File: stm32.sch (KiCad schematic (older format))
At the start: 39 parts, among them J2 MINI-USB-5P-3400020P1, J3 Conn_02x05_Odd_Even, U1 STM32F767VITx, U30 LM2937, X1 8MHz, X2 32.768K

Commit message: fix usb
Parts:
- removed J2: MINI-USB-5P-3400020P1, Connector_USB:USB_Micro-B_Molex-105133-0031, symbol BOSCH_154_PIN:MINI-USB-5P-3400020P1
- removed R102: 10K, Resistor_SMD:R_0805_2012Metric_Pad1.15x1.40mm_HandSolder, symbol ME7_Universal-rescue:R-adc_amp_dividor-cache-ME7_Universal-rescue
- removed R103: 680, Resistor_SMD:R_0805_2012Metric_Pad1.15x1.40mm_HandSolder, symbol ME7_Universal-rescue:R-adc_amp_dividor-cache-ME7_Universal-rescue
- added J2: USB_B_Micro, symbol Connector:USB_B_Micro
- added R102: 10k, symbol Device:R
- added R103: 680, symbol Device:R
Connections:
- wire segments 74 -> 75
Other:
- moved on the sheet: C75, D17, R100
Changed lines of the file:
@@
-$EndComp
-$Comp
-L BOSCH_154_PIN:MINI-USB-5P-3400020P1 J2
-U 1 1 52D197D7
-P 11600 4250
-F 0 "J2" H 11325 4600 60  0000 C CNN
-F 1 "MINI-USB-5P-3400020P1" H 11600 4700 60  0001 C CNN
-F 2 "Connector_USB:USB_Micro-B_Molex-105133-0031" V 430 1700 60  0001 C CNN
-F 3 "" H 11600 4250 60  0001 C CNN
-F 4 "stm32f407_board" H 11950 1275 60  0001 C CNN "PageName"
-F 5 "MOUSER" H -6050 -2300 50  0001 C CNN "VEND"
-F 6 "MOLEX" H -6050 -2300 50  0001 C CNN "Manufacturer"
-F 7 "105133-0031" H -6050 -2300 50  0001 C CNN "Part #"
-F 8 "538-105133-0031" H -6050 -2300 50  0001 C CNN "VEND#"
-	1    11600 4250
-	1    0    0    -1
 $EndComp
 $Comp
 L power:GND #PWR0141
 U 1 1 5CE96D9C
-P 12100 4600
-F 0 "#PWR0141" H 12100 4600 30  0001 C CNN
-F 1 "GND" H 12100 4530 30  0001 C CNN
-F 2 "" H 12100 4600 60  0000 C CNN
-F 3 "" H 12100 4600 60  0000 C CNN
-	1    12100 4600
+P 11500 4750
+F 0 "#PWR0141" H 11500 4750 30  0001 C CNN
+F 1 "GND" H 11500 4680 30  0001 C CNN
+F 2 "" H 11500 4750 60  0000 C CNN
+F 3 "" H 11500 4750 60  0000 C CNN
+	1    11500 4750
 	1    0    0    -1
 $EndComp
@@
 L power:GND #PWR0144
 U 1 1 5C5BFED2
-P 12950 5000
-F 0 "#PWR0144" H 12950 5000 30  0001 C CNN
-F 1 "GND" H 12950 4930 30  0001 C CNN
-F 2 "" H 12950 5000 60  0001 C CNN
-F 3 "" H 12950 5000 60  0001 C CNN
-	1    12950 5000
-	1    0    0    -1
-$EndComp
-Text Notes 12800 5800 0    60   ~ 12
+P 12950 5050
+F 0 "#PWR0144" H 12950 5050 30  0001 C CNN
+F 1 "GND" H 12950 4980 30  0001 C CNN
+F 2 "" H 12950 5050 60  0001 C CNN
+F 3 "" H 12950 5050 60  0001 C CNN
+	1    12950 5050
+	1    0    0    -1
+$EndComp
+Text Notes 11750 6650 0    60   ~ 12
 SWD
 Text Label 12100 6300 0    60   ~ 12
@@
 Text Notes 12450 5250 0    60   ~ 12
 diodes schottky 20V 1A SD0805S020S1R0
-Text Label 13450 4300 0    60   ~ 12
+Text Label 13450 4400 0    60   ~ 12
 PA10
-Text Label 14250 4000 0    60   ~ 12
+Text Label 14150 4000 0    60   ~ 12
 PA9
 Text HLabel 6600 2000 2    60   Input ~ 12
@@
 Text HLabel 14150 3400 0    60   Input ~ 12
 5V
-Text HLabel 12200 4400 2    60   Input ~ 12
+Text HLabel 11500 4650 2    60   Input ~ 12
 GND
-Text Label 11800 4500 0    60   ~ 12
+Text Label 11400 4700 2    60   ~ 12
 shield
 Wire Wire Line
@@
 Wire Wire Line
 	12300 3800 12400 3800
-$Comp
-L ME7_Universal-rescue:R-adc_amp_dividor-cache-ME7_Universal-rescue R?
-U 1 1 5C7B03F9
-P 15800 3400
-AR Path="/5C7B03F9" Ref="R?"  Part="1"
-AR Path="/5D0250FB/5C7B03F9" Ref="R103"  Part="1"
-F 0 "R103" V 15700 3400 40  0000 C CNN
-F 1 "680" V 15800 3400 40  0000 C CNN
-F 2 "Resistor_SMD:R_0805_2012Metric_Pad1.15x1.40mm_HandSolder" V 15730 3400 30  0001 C CNN
-F 3 "" H 15800 3400 30  0000 C CNN
-	1    15800 3400
-	0    1    1    0
-$EndComp
 Wire Wire Line
 	14900 3400 15200 3400
@@
 L Power_Protection:ESDA6V1BC6 D17
 U 1 1 5C850928
-P 12950 4700
-F 0 "D17" H 13280 4746 50  0000 L CNN
-F 1 "ESDA6V1BC6" H 13280 4655 50  0000 L CNN
-F 2 "Package_TO_SOT_SMD:SOT-23-6" H 12950 4350 50  0001 C CNN
-F 3 "http://www.st.com/content/ccc/resource/technical/document/datasheet/21/07/21/e3/a8/df/42/a2/CD00001906.pdf/files/CD00001906.pdf/jcr:content/translations/en.CD00001906.pdf" V 12950 4700 50  0001 C CNN
-	1    12950 4700
-	1    0    0    -1
-$EndComp
-Text Label 13450 4100 0    60   ~ 12
+P 12950 4750
+F 0 "D17" H 13280 4796 50  0000 L CNN
+F 1 "ESDA6V1BC6" H 13280 4705 50  0000 L CNN
+F 2 "Package_TO_SOT_SMD:SOT-23-6" H 12950 4400 50  0001 C CNN
+F 3 "http://www.st.com/content/ccc/resource/technical/document/datasheet/21/07/21/e3/a8/df/42/a2/CD00001906.pdf/files/CD00001906.pdf/jcr:content/translations/en.CD00001906.pdf" V 12950 4750 50  0001 C CNN
+	1    12950 4750
+	1    0    0    -1
+$EndComp
+Text Label 13450 4300 0    60   ~ 12
 PA11
 Text Label 13450 4200 0    60   ~ 12
@@
 	11800 4200 13050 4200
 Wire Wire Line
-	11800 4100 12850 4100
-Wire Wire Line
-	11800 4300 13150 4300
-Wire Wire Line
 	11875 4000 12750 4000
-Wire Wire Line
-	12750 4400 12750 4000
 Connection ~ 12750 4000
-Wire Wire Line
-	12850 4400 12850 4100
-Connection ~ 12850 4100
-Wire Wire Line
-	12850 4100 13450 4100
-Wire Wire Line
-	13050 4400 13050 4200
 Connection ~ 13050 4200
 Wire Wire Line
 	13050 4200 13450 4200
-Wire Wire Line
-	13150 4400 13150 4300
-Connection ~ 13150 4300
-Wire Wire Line
-	13150 4300 13450 4300
-$Comp
-L ME7_Universal-rescue:R-adc_amp_dividor-cache-ME7_Universal-rescue R?
-U 1 1 5C920125
-P 14000 4000
-AR Path="/5C920125" Ref="R?"  Part="1"
-AR Path="/5D0250FB/5C920125" Ref="R102"  Part="1"
-F 0 "R102" V 13900 4000 40  0000 C CNN
-F 1 "10K" V 14000 4000 40  0000 C CNN
-F 2 "Resistor_SMD:R_0805_2012Metric_Pad1.15x1.40mm_HandSolder" V 13930 4000 30  0001 C CNN
-F 3 "" H 14000 4000 30  0000 C CNN
-	1    14000 4000
-	0    1    1    0
-$EndComp
-Text Label 12150 4100 0    60   ~ 0
+Text Label 12150 4300 0    60   ~ 0
 D-
 Text Label 12150 4200 0    60   ~ 0
@@
 Wire Wire Line
 	13150 4000 13750 4000
-Wire Wire Line
-	11800 4400 12100 4400
-Wire Wire Line
-	12100 4400 12100 4600
-Connection ~ 12100 4400
-Wire Wire Line
-	12100 4400 12200 4400
 Wire Wire Line
 	14300 3400 14150 3400
@@
 $EndComp
 Wire Wire Line
-	11600 4650 11800 4650
-Wire Wire Line
-	11800 4500 11800 4650
-Wire Wire Line
-	11800 4650 11800 4750
-Connection ~ 11800 4650
+	11200 4750 11400 4750
+Wire Wire Line
+	11400 4600 11400 4750
+Wire Wire Line
+	11400 4750 11400 4850
+Connection ~ 11400 4750
 $Comp
 L power:GND #PWR0138
 U 1 1 5C5BFED7
-P 11600 4950
-F 0 "#PWR0138" H 11600 4950 30  0001 C CNN
-F 1 "GND" H 11600 4880 30  0001 C CNN
-F 2 "" H 11600 4950 60  0001 C CNN
-F 3 "" H 11600 4950 60  0001 C CNN
-	1    11600 4950
+P 11200 5050
+F 0 "#PWR0138" H 11200 5050 30  0001 C CNN
+F 1 "GND" H 11200 4980 30  0001 C CNN
+F 2 "" H 11200 5050 60  0001 C CNN
+F 3 "" H 11200 5050 60  0001 C CNN
+	1    11200 5050
 	1    0    0    -1
 $EndComp
@@
 L Device:R R100
 U 1 1 5D0251FB
-P 11600 4800
-F 0 "R100" V 11680 4800 50  0000 C CNN
-F 1 "100k" V 11600 4800 50  0000 C CNN
-F 2 "Resistor_SMD:R_0805_2012Metric_Pad1.15x1.40mm_HandSolder" H 11600 4800 60  0001 C CNN
-F 3 "" H 11600 4800 60  0001 C CNN
-F 4 "stm32f407_board" H 11950 1175 60  0001 C CNN "PageName"
-F 5 "MOUSER" H -6050 -2300 50  0001 C CNN "VEND"
-	1    11600 4800
+P 11200 4900
+F 0 "R100" V 11280 4900 50  0000 C CNN
+F 1 "100k" V 11200 4900 50  0000 C CNN
+F 2 "Resistor_SMD:R_0805_2012Metric_Pad1.15x1.40mm_HandSolder" H 11200 4900 60  0001 C CNN
+F 3 "" H 11200 4900 60  0001 C CNN
+F 4 "stm32f407_board" H 11550 1275 60  0001 C CNN "PageName"
+F 5 "MOUSER" H -6450 -2200 50  0001 C CNN "VEND"
+	1    11200 4900
 	-1   0    0    -1
 $EndComp
@@
 L power:GND #PWR0140
 U 1 1 5D0251FA
-P 11800 5050
-F 0 "#PWR0140" H 11800 5050 30  0001 C CNN
-F 1 "GND" H 11800 4980 30  0001 C CNN
-F 2 "" H 11800 5050 60  0001 C CNN
-F 3 "" H 11800 5050 60  0001 C CNN
-	1    11800 5050
+P 11400 5150
+F 0 "#PWR0140" H 11400 5150 30  0001 C CNN
+F 1 "GND" H 11400 5080 30  0001 C CNN
+F 2 "" H 11400 5150 60  0001 C CNN
+F 3 "" H 11400 5150 60  0001 C CNN
+	1    11400 5150
 	1    0    0    -1
 $EndComp
@@
 L Device:C C75
 U 1 1 5D0251F9
-P 11800 4900
-F 0 "C75" H 11850 5000 50  0000 L CNN
-F 1 "100nF" H 11850 4800 50  0000 L CNN
-F 2 "Capacitor_SMD:C_0805_2012Metric_Pad1.15x1.40mm_HandSolder" V 430 1650 60  0001 C CNN
-F 3 "" H 11800 4900 60  0001 C CNN
-F 4 "stm32f407_board" H 11950 1225 60  0001 C CNN "PageName"
-F 5 "KEMET" H -6050 -2300 50  0001 C CNN "Manufacturer"
-F 6 "C1206C104J3GECAUTO" H -6050 -2300 50  0001 C CNN "Part #"
-F 7 "MOUSER" H -6050 -2300 50  0001 C CNN "VEND"
-F 8 "80-C1206C104J3GECAUT" H -6050 -2300 50  0001 C CNN "VEND#"
-	1    11800 4900
+P 11400 5000
+F 0 "C75" H 11450 5100 50  0000 L CNN
+F 1 "100nF" H 11450 4900 50  0000 L CNN
+F 2 "Capacitor_SMD:C_0805_2012Metric_Pad1.15x1.40mm_HandSolder" V 30  1750 60  0001 C CNN
+F 3 "" H 11400 5000 60  0001 C CNN
+F 4 "stm32f407_board" H 11550 1325 60  0001 C CNN "PageName"
+F 5 "KEMET" H -6450 -2200 50  0001 C CNN "Manufacturer"
+F 6 "C1206C104J3GECAUTO" H -6450 -2200 50  0001 C CNN "Part #"
+F 7 "MOUSER" H -6450 -2200 50  0001 C CNN "VEND"
+F 8 "80-C1206C104J3GECAUT" H -6450 -2200 50  0001 C CNN "VEND#"
+	1    11400 5000
 	1    0    0    -1
 $EndComp
@@
 Wire Wire Line
 	6750 2650 6750 3550
+$Comp
+L Connector:USB_B_Micro J2
+U 1 1 5CDEB9A6
+P 11500 4200
+F 0 "J2" H 11557 4667 50  0000 C CNN
+F 1 "USB_B_Micro" H 11557 4576 50  0000 C CNN
+F 2 "" H 11650 4150 50  0001 C CNN
+F 3 "~" H 11650 4150 50  0001 C CNN
+	1    11500 4200
+	1    0    0    -1
+$EndComp
+Wire Wire Line
+	11500 4750 11500 4600
+Wire Wire Line
+	13150 4450 13150 4400
+Wire Wire Line
+	13150 4400 13450 4400
+Wire Wire Line
+	13450 4300 12850 4300
+Wire Wire Line
+	12850 4300 12850 4450
+Connection ~ 12850 4300
+Wire Wire Line
+	12850 4300 11800 4300
+Wire Wire Line
+	13050 4200 13050 4450
+Wire Wire Line
+	12750 4000 12750 4450
+Wire Wire Line
+	11800 4400 13150 4400
+Connection ~ 13150 4400
+$Comp
+L Device:R R102
+U 1 1 5CE17917
+P 13900 4000
+F 0 "R102" V 14000 4000 50  0000 C CNN
+F 1 "10k" V 13900 4000 50  0000 C CNN
+F 2 "" V 13830 4000 50  0001 C CNN
+F 3 "~" H 13900 4000 50  0001 C CNN
+	1    13900 4000
+	0    1    1    0
+$EndComp
+$Comp
+L Device:R R103
+U 1 1 5CE182F0
+P 15800 3400
+F 0 "R103" V 15900 3400 50  0000 C CNN
+F 1 "680" V 15800 3400 50  0000 C CNN
+F 2 "" V 15730 3400 50  0001 C CNN
+F 3 "~" H 15800 3400 50  0001 C CNN
+	1    15800 3400
+	0    1    1    0
+$EndComp
+Wire Wire Line
+	15550 3400 15650 3400
+Wire Wire Line
+	15950 3400 16050 3400
+Wire Wire Line
+	14150 4000 14050 4000
 $EndSCHEMATC

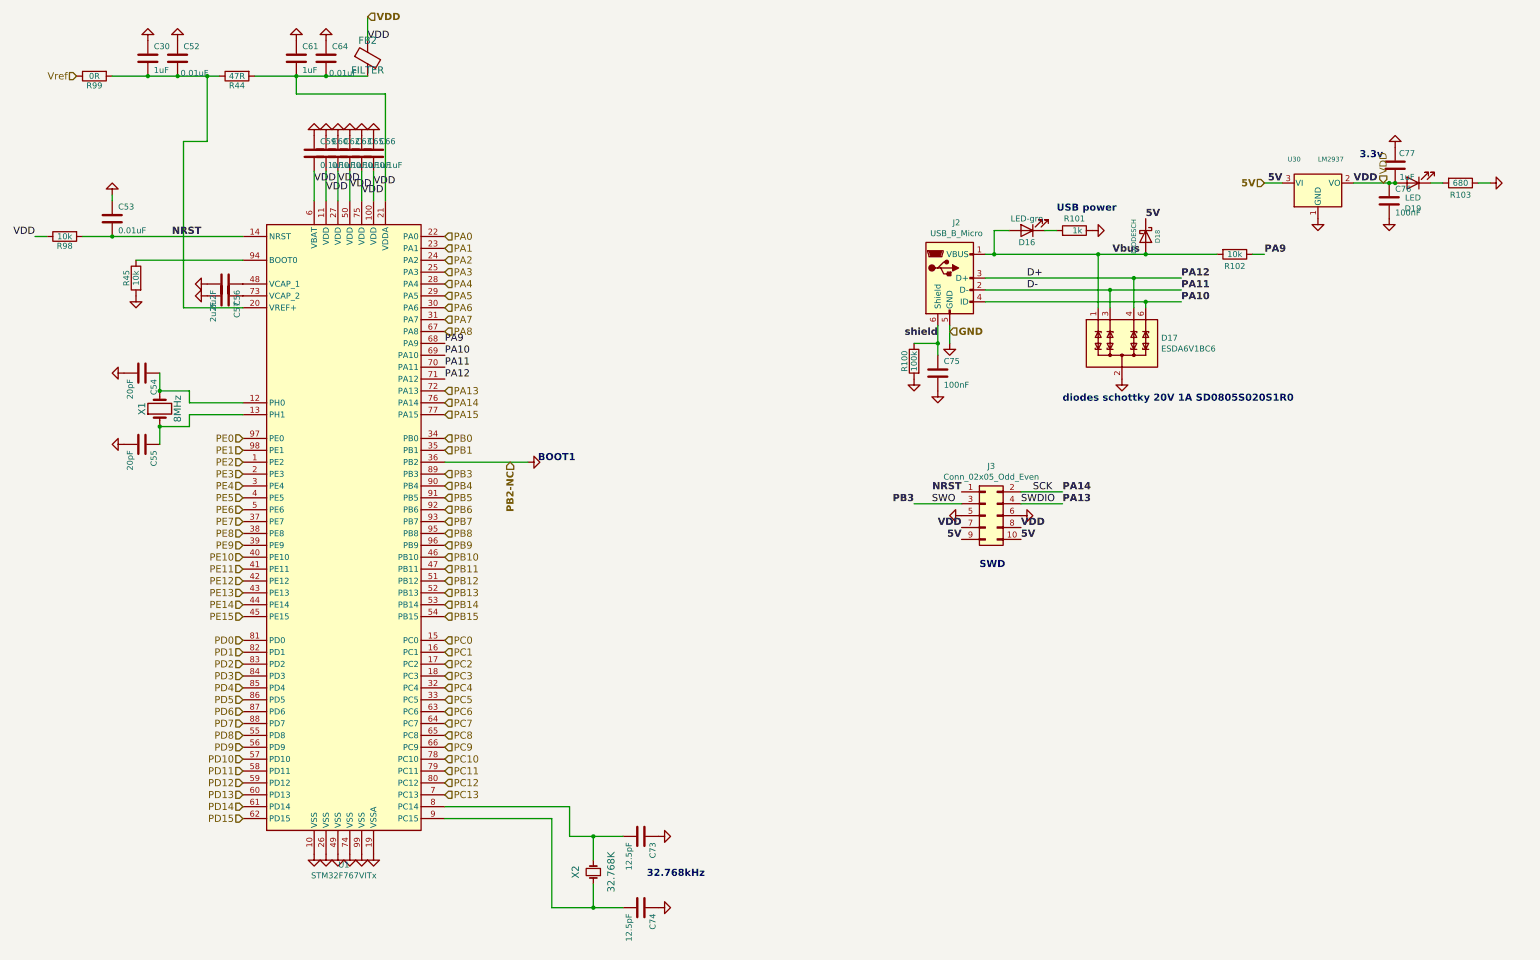
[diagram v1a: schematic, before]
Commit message: Latest schematics
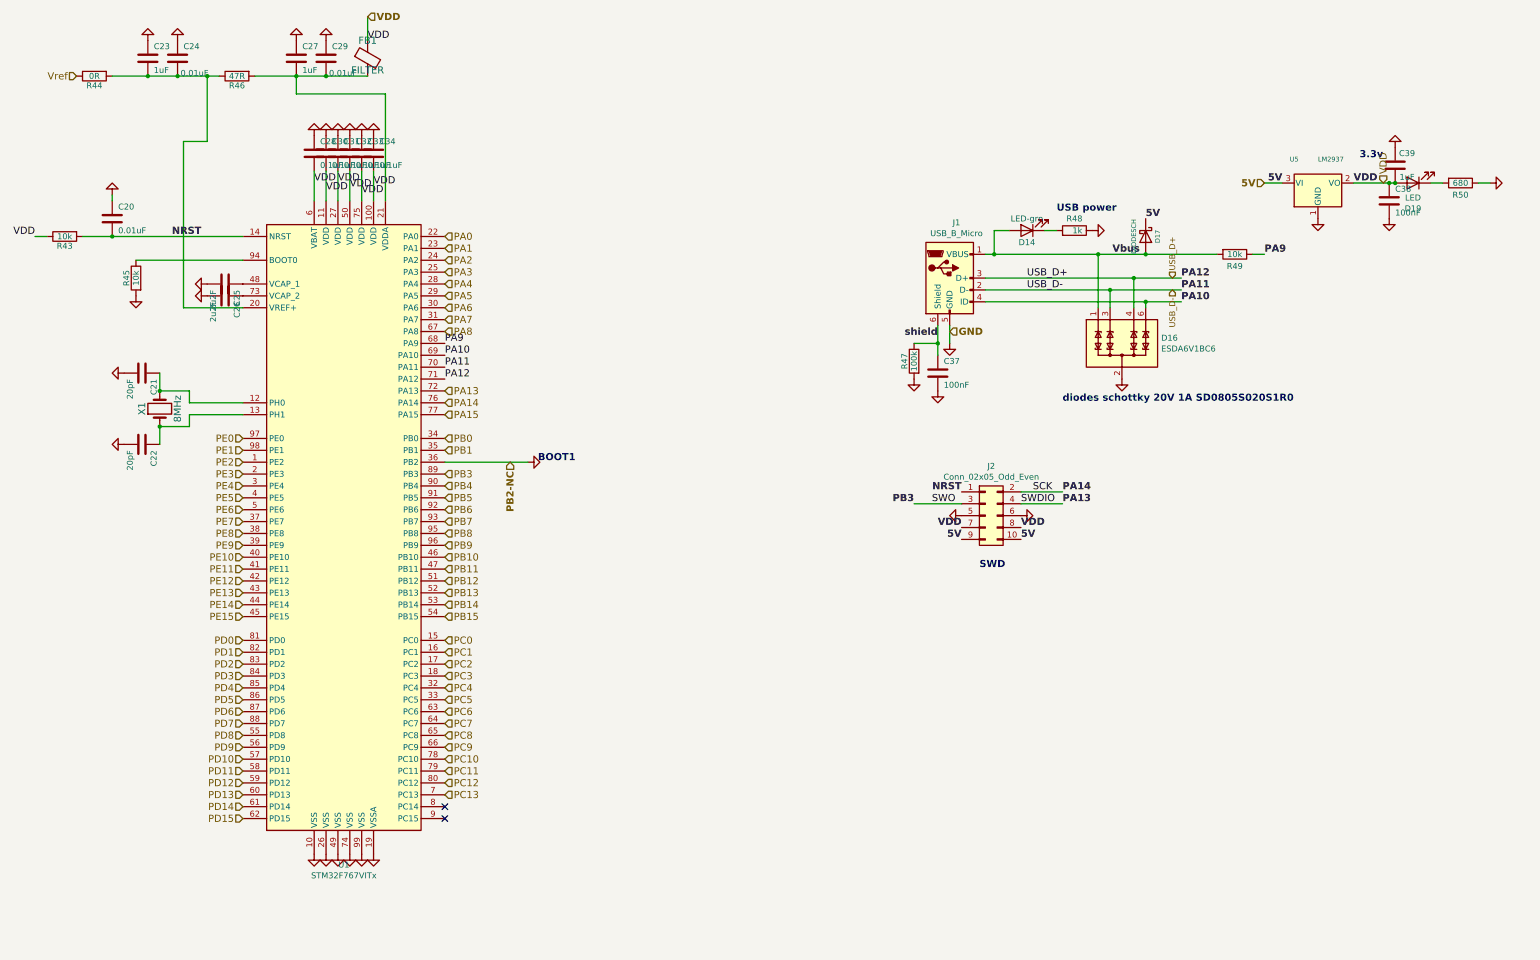
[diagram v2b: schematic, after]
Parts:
- removed C73, C74: 12.5pF, Capacitor_SMD:C_0805_2012Metric_Pad1.15x1.40mm_HandSolder, symbol Device:C
- removed X2: 32.768K, Crystal:Crystal_SMD_MicroCrystal_CC7V-T1A-2Pin_3.2x1.5mm_HandSoldering, symbol Device:Crystal_Small
- J1: renamed from J2; footprint (none) -> Connector_USB:USB_Micro-B_Molex-105133-0031
- R49: renamed from R102; footprint (none) -> Resistor_SMD:R_0603_1608Metric_Pad1.05x0.95mm_HandSolder
- R50: renamed from R103; footprint (none) -> Resistor_SMD:R_0603_1608Metric_Pad1.05x0.95mm_HandSolder
- renumbered C53 to C20, C54 to C21, C55 to C22, C30 to C23, C52 to C24, C56 to C25, C57 to C26, C61 to C27, C59 to C28, C64 to C29, C60 to C30, C62 to C31, C63 to C32, C65 to C33, C66 to C34, C75 to C37, C76 to C38, C77 to C39, D16 to D14, D17 to D16, D18 to D17, FB2 to FB1, J3 to J2, R98 to R43, R99 to R44, R44 to R46, R100 to R47, R101 to R48, U30 to U5
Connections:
- net D+ renamed USB_D+
- net D- renamed USB_D-
- no-connect marks 0 -> 2
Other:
- note removed: "32.768kHz"

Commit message: changed to lm2937 ldo (#20)
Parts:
- U5: symbol Regulator_Linear:LD1117S33TR_SOT223 -> Regulator_Linear:LM2937xMP
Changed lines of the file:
@@
-EESchema Schematic File Version 4
+EESchema Schematic File Version 5
 LIBS:microRusEfi-cache
 EELAYER 29 0
@@
 $EndComp
 $Comp
-L Regulator_Linear:LD1117S33TR_SOT223 U5
+L Regulator_Linear:LM2937xMP U5
 U 1 1 5D0251EC
 P 14600 3400

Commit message: Update of returning faults each pull (#21)
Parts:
- C20, C21, C22, C23, C24, C25, C26, C27, C28, C29, C30, C31, C32, C33, C34, C37, C38, C39, D14, D17: footprint Capacitor_SMD:C_0805_2012Metric_Pad1.15x1.40mm_HandSolder -> Capacitor_SMD:C_0603_1608Metric_Pad1.05x0.95mm_HandSolder
- D19: footprint LED_SMD:LED_1206_3216Metric_Pad1.42x1.75mm_HandSolder -> LED_SMD:LED_0603_1608Metric_Pad1.05x0.95mm_HandSolder
- FB1, R43, R44, R45, R46, R47, R48: footprint Resistor_SMD:R_0805_2012Metric_Pad1.15x1.40mm_HandSolder -> Resistor_SMD:R_0603_1608Metric_Pad1.05x0.95mm_HandSolder

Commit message: manual sync with 960
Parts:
- removed R49: 10k, Resistor_SMD:R_0603_1608Metric_Pad1.05x0.95mm_HandSolder, symbol Device:R
- added C36: 1uF, Capacitor_SMD:C_0603_1608Metric_Pad1.05x0.95mm_HandSolder, symbol Device:C
- C20, C24, C29: value 0.01uF -> 10nF; MFG,MFG# AVX,08051C103JAT2A -> (none); VEND1,VEND1# DIGI,478-3745-6-ND -> (none)
- C21, C22: Manufacturer KEMET -> (none); Part # C1206X200M5HACTU -> (none); VEND MOUSER -> (none); VEND# 80-C1206X200M5HACTU -> (none)
- C23, C27: MFG,MFG# TDK,C2012X7S2A105K125AB -> (none); VEND1,VEND1# DIGI,445-5205-6-ND -> (none)
- C25, C26: value 2u2F -> 2.2uF; MFG,MFG# TDK,CGA4J3X5R1H225K125AB -> (none); VEND1,VEND1# DIGI,445-7880-1-ND -> (none)
- C28, C30, C31, C32, C33, C34: value 0.1uF -> 10nF; MFG,MFG# AVX,08055C104KAT2A -> (none); VEND1,VEND1# DIGI,478-1395-1-ND -> (none)
- C37, C38: Manufacturer KEMET -> (none); Part # C1206C104J3GECAUTO -> (none); VEND MOUSER -> (none); VEND# 80-C1206C104J3GECAUT -> (none)
- C39: value 1uF -> 15uF; footprint Capacitor_SMD:C_0603_1608Metric_Pad1.05x0.95mm_HandSolder -> Capacitor_SMD:C_1206_3216Metric_Pad1.42x1.75mm_HandSolder; Manufacturer WURTH -> (none); Part # 885012208064 -> TAJA156M010RNJ; VEND MOUSER -> (none); VEND# 710-885012208064 -> (none)
- D14: value LED-grn -> LED-green
- FB1: MFG,MFG# Murata,BLM21PG221SN1D -> (none); Part Manufacturer MURATA -> (none); VEND1,VEND1# DIGI,490-1054-6-ND -> (none)
- J2: footprint (none) -> Connector_PinSocket_2.54mm:PinSocket_2x05_P2.54mm_Vertical_SMD
- R43, R44, R45, R46: MFG,MFG# BOURNS,CR0805-FX-1002ELF -> (none); VEND1,VEND1# DIGI,CR0805-FX-1002ELFCT-ND -> (none)
- R48: VEND MOUSER -> (none)
- U1: Part # (none) -> 511-STM32F767VIT6
- U5: Manufacturer ST MICRO -> (none); Part # LD1117S50TR -> 926-LM2937IMP3.3NOPB; VEND# 511-LD1117S50 -> (none)
- X1: Manufacturer NDK -> (none)
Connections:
- wire segments 65 -> 70
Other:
- moved on the sheet: C39
